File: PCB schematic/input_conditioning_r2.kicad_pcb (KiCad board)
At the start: 4 copper layers, 194.5 x 113 mm, 57 parts, among them J1 Conn_01x10_Socket, J2 Conn_01x02_Socket, J3 Conn_Coaxial_x2, J7 Conn_01x08_Socket, SW1 Shifting, SW2 Scaling, SW3 Trigger, U1 OPA2365AID, U2 OPA2365AID

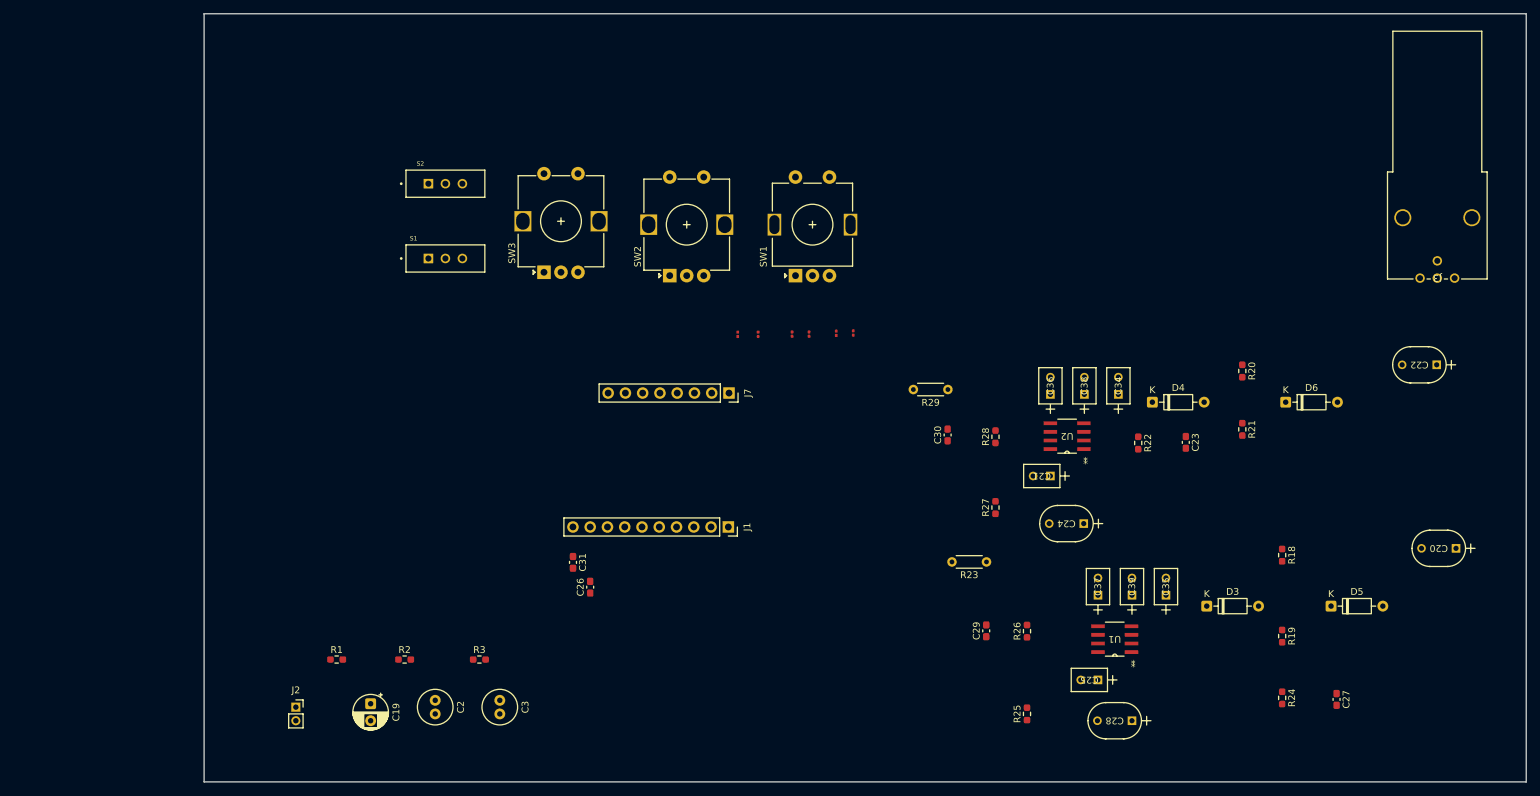
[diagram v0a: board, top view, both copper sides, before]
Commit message: pcb initial complete revision
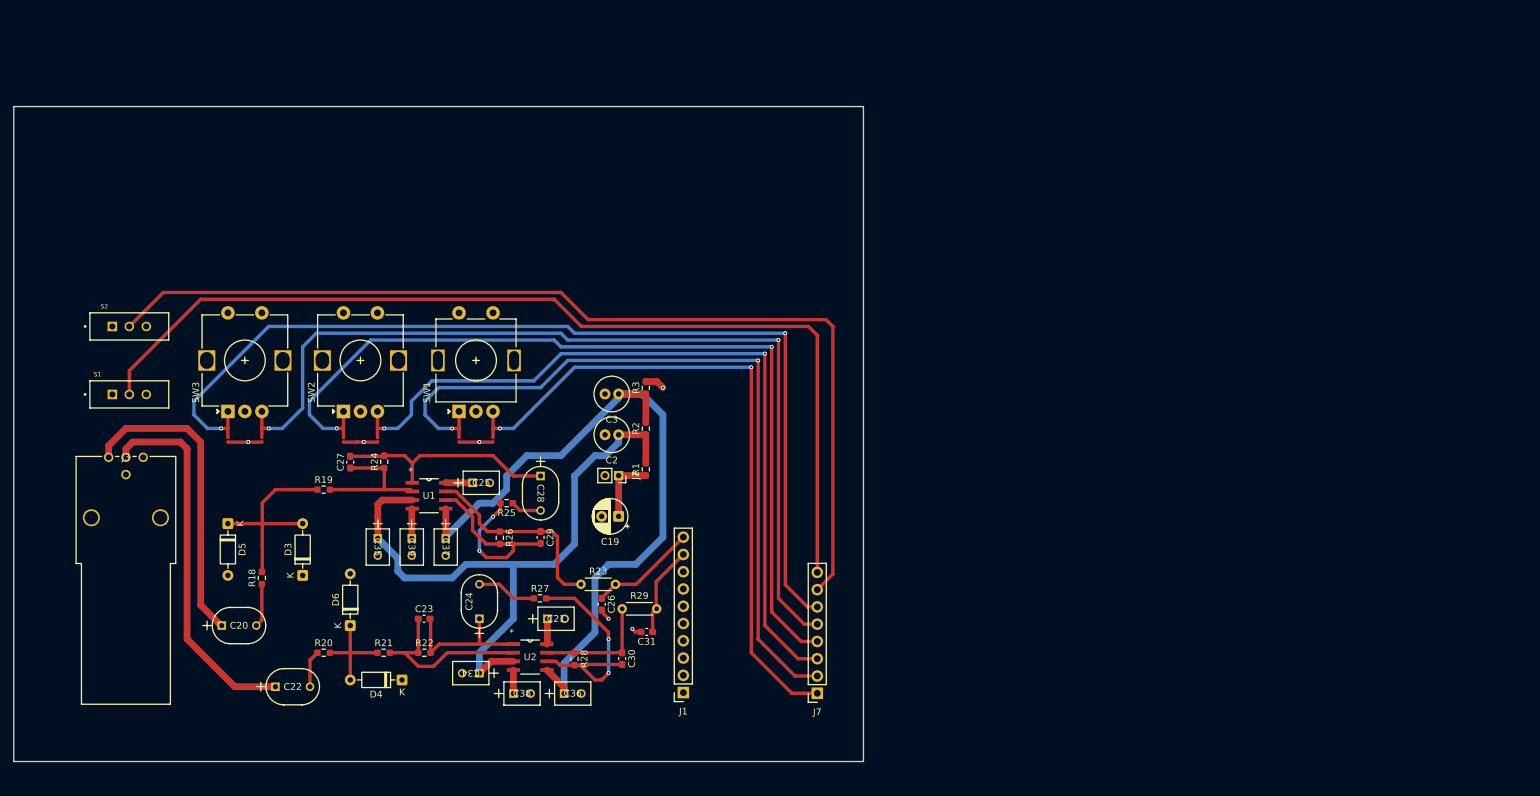
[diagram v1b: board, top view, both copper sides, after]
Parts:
- moved J3 194.7 mm to (56.0, 113.3), turned to 0 degrees
- moved C20 181.9 mm to (70.1, 138.0), turned to 0 degrees
- moved C22 177.3 mm to (78.0, 147.0), turned to 0 degrees
- moved D5 162.7 mm to (71.0, 123.0), turned to -90 degrees
- moved R18 150.1 mm to (76.0, 131.0), turned to 90 degrees
- moved C27 149.2 mm to (89.0, 114.0), turned to 90 degrees
- moved R19 142.6 mm to (85.1, 118.0), turned to 0 degrees
- moved D6 141.5 mm to (89.0, 138.0), turned to 90 degrees
- moved R20 141.4 mm to (85.1, 142.0), turned to 0 degrees
- moved R24 136.6 mm to (94.0, 113.9), turned to 90 degrees
- moved D3 133.1 mm to (82.0, 130.6), turned to 90 degrees
- moved R21 130.5 mm to (93.9, 142.0), turned to 0 degrees
- moved D4 117.7 mm to (96.6, 146.0), turned to 180 degrees
- moved C35 116.3 mm to (93.0, 125.2), turned to -90 degrees
- moved C23 115.0 mm to (99.9, 137.0), turned to 0 degrees
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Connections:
- D3 pad 2: Net-(D3-A) -> /Real Signal Processing 1/ac_coupled
- D4 pad 2: Net-(D4-A) -> /Real Signal Processing 2/ac_coupled
- D5 pad 1: Net-(D3-A) -> /Real Signal Processing 1/ac_coupled
- D6 pad 1: Net-(D4-A) -> /Real Signal Processing 2/ac_coupled
- J1 pad 10: /output_2 -> /output_1
- J1 pad 9: /output_1 -> /output_2
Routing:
- net +3V3: track 0.00 -> 161.2 mm, vias 0 -> 3
- net Net-(J7-Pin_7): track 0.00 -> 147.3 mm
- net Net-(J7-Pin_6): track 0.00 -> 146.6 mm, vias 0 -> 2
- net Net-(J7-Pin_8): track 0.00 -> 146.1 mm
- net Net-(J7-Pin_5): track 0.00 -> 136.6 mm, vias 0 -> 2
- net Net-(J7-Pin_4): track 0.00 -> 131.3 mm, vias 0 -> 2
- net Net-(J7-Pin_3): track 0.00 -> 116.2 mm, vias 0 -> 2
- net Net-(J7-Pin_2): track 0.00 -> 115.1 mm, vias 0 -> 2
- net /+1V25: track 0.00 -> 110.2 mm
- net Net-(J7-Pin_1): track 0.00 -> 99.7 mm, vias 0 -> 2
- net +2V5: track 0.00 -> 96.5 mm
- net /input_2: track 0.00 -> 55.0 mm
- net /input_1: track 0.00 -> 45.5 mm
- net /Real Signal Processing 2/s2_in: track 0.00 -> 34.0 mm, vias 0 -> 2
- net /Real Signal Processing 1/s1_out: track 0.00 -> 33.1 mm
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- added copper zone on In2.Cu, net +5V
- added copper zone on In1.Cu, net GND
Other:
- board size 194.5 x 113 mm -> 125 x 96.4 mm
- board text added: "pico"
- board text removed: "BNC"
